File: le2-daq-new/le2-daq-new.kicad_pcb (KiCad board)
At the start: 2 copper layers, 161.3 x 88.4 mm, 11 parts, among them J1 PCIE_CONN, J2 PCIE_CONN, J3 PCIE_CONN, J4 PCIE_CONN, J5 Conn_01x02_Male, J6 TEST-POINT, J7 TEST-POINT, SW1 EN_HIGH, U1 ESP32-DEVKITC-32D

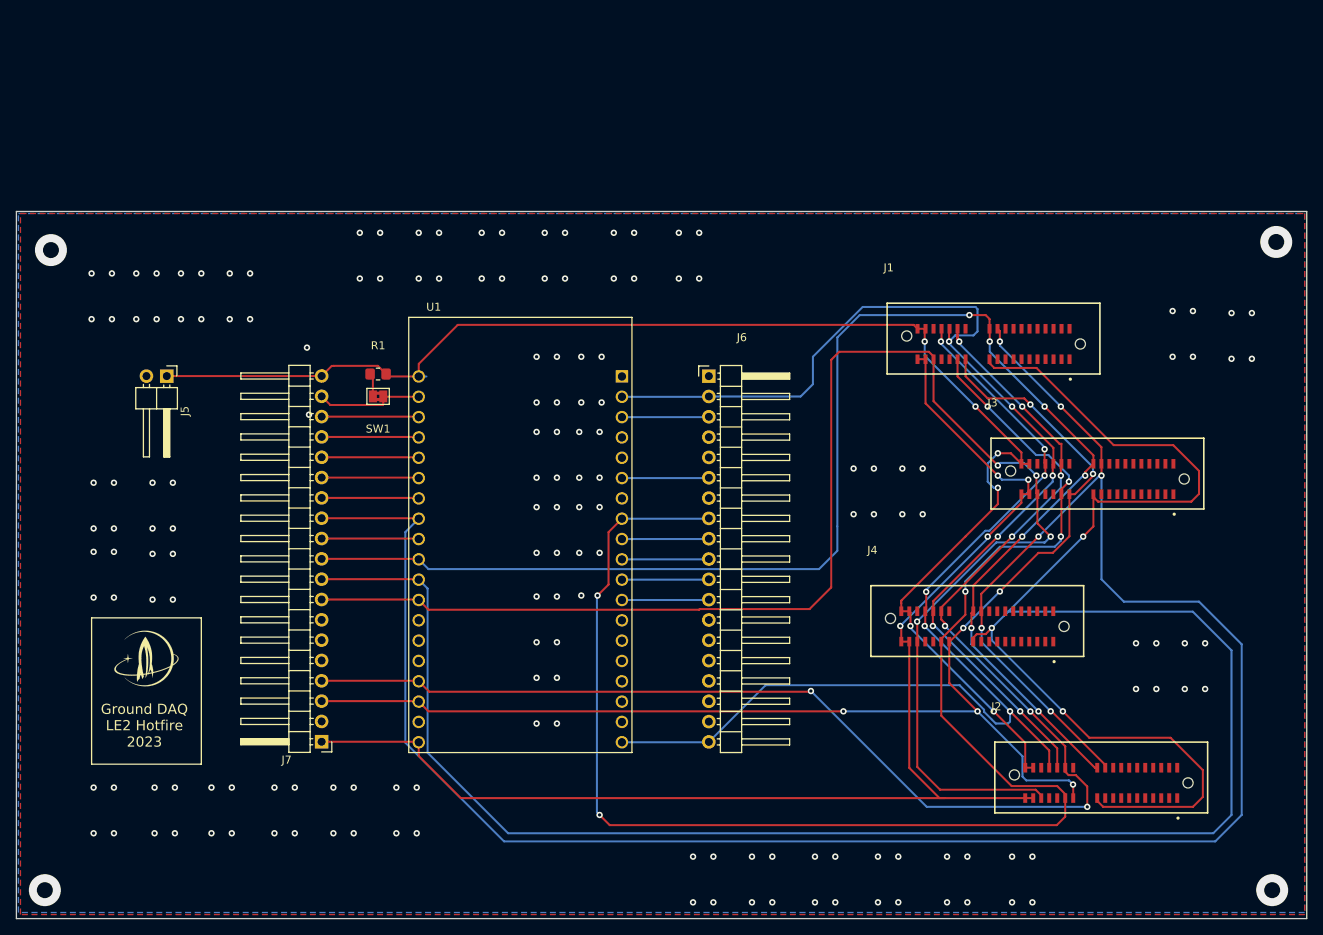
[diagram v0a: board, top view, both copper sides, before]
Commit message: done with daq layout FRFRFRF
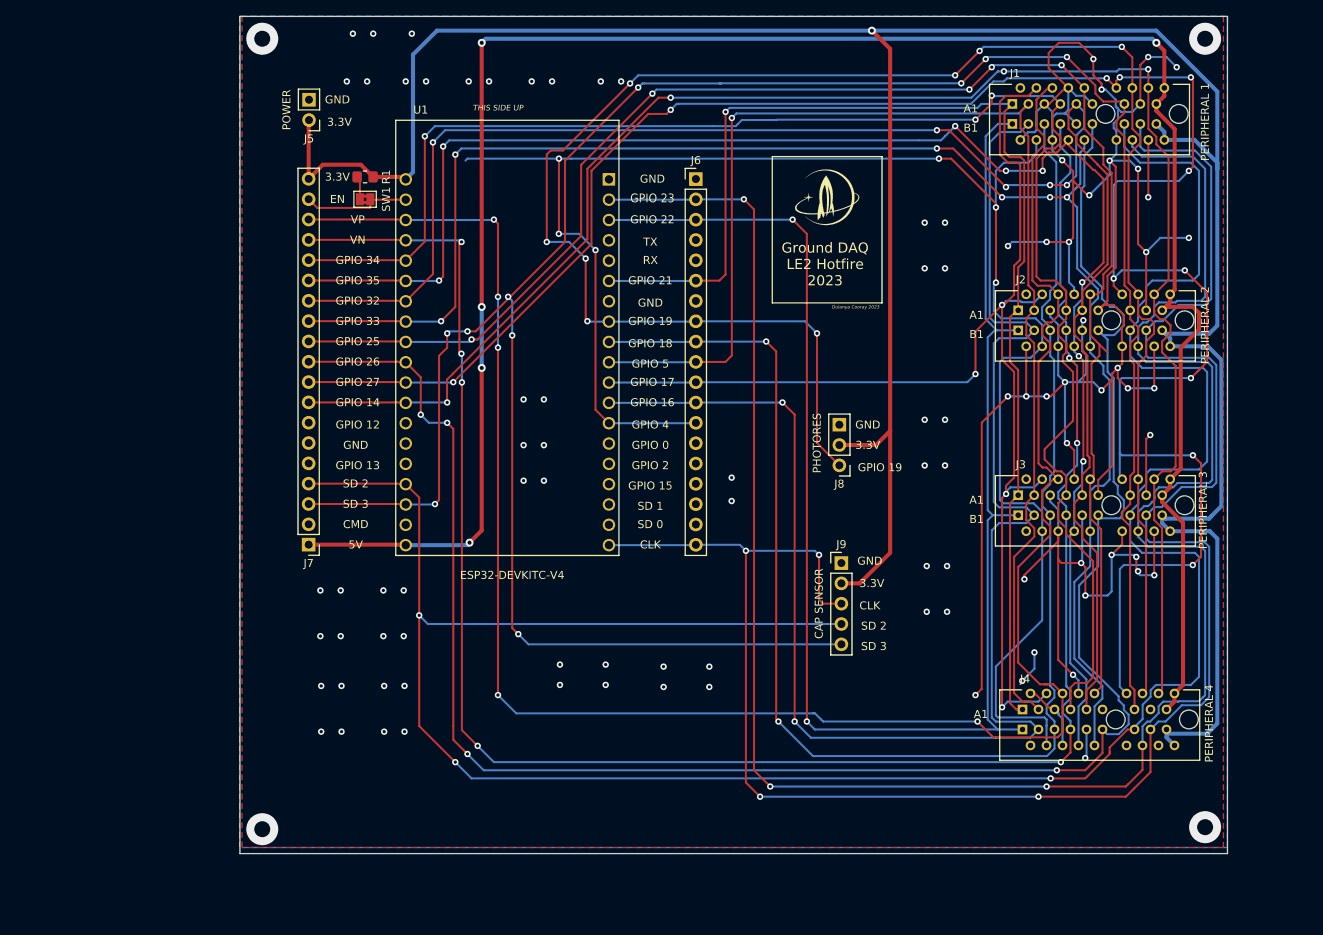
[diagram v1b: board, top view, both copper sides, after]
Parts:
- added J8: Conn_01x03_Male, Connector_PinHeader_2.54mm:PinHeader_1x03_P2.54mm_Vertical, F.Cu at (157.0, 89.4)
- added J9: Conn_01x05_Male, Connector_PinHeader_2.54mm:PinHeader_1x05_P2.54mm_Vertical, F.Cu at (157.2, 101.6)
- J1, J2, J3, J4: footprint PCIE-LP-01-01-F-DV-A-TR:SAMTEC_PCIE-LP-01-01-F-DV-A-TR -> AMPHENOL-PCIE-Socket:AMPHENOL_10018784-10210TLF
- J5: footprint Connector_PinHeader_2.54mm:PinHeader_1x02_P2.54mm_Horizontal -> Connector_PinHeader_2.54mm:PinHeader_1x02_P2.54mm_Vertical
- J6, J7: footprint Connector_PinHeader_2.54mm:PinHeader_1x19_P2.54mm_Horizontal -> Connector_PinHeader_2.54mm:PinHeader_1x19_P2.54mm_Vertical
- SW1: value EN_HIGH -> SW_Push
- moved G*** 102.8 mm to (155.4, 55.9)
- moved J2 57.8 mm to (191.0, 71.3)
- moved J5 36.6 mm to (90.7, 46.2), turned to 180 degrees
- moved J1 32.0 mm to (190.2, 45.5)
- moved J6 24.7 mm to (139.0, 53.6)
- moved SW1 24.7 mm to (97.7, 56.1)
- moved J7 24.7 mm to (90.6, 99.3)
- moved R1 24.7 mm to (97.7, 53.3)
- moved U1 24.7 mm to (115.5, 73.4)
- moved J4 20.8 mm to (191.5, 121.2)
- moved J3 3.71 mm to (191.0, 94.4)
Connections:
- J1 pad A01: (no net) -> RL SDA
- J1 pad A02: (no net) -> GND
- J1 pad A03: (no net) -> TC SDO
- J1 pad A04: (no net) -> TC SDI
- J1 pad A05: (no net) -> GND
- J1 pad A06: (no net) -> HX 1
- J1 pad A07: (no net) -> HX 3
- J1 pad A08: (no net) -> GND
- J1 pad A09: (no net) -> HX 5
- J1 pad A10: GND -> HX 7
- J1 pad A11: HX CLK -> GND
- J1 pad A12: CAP 2 -> HX CLK
- J1 pad A13: PHOTORES -> CAP 2
- J1 pad A14: GND -> PHOTORES
- J1 pad B01: (no net) -> RL SCL
- J1 pad B02: (no net) -> GND
- J1 pad B03: (no net) -> TC1 CS
- J1 pad B04: (no net) -> TC2 CS
- J1 pad B05: (no net) -> TC CLK
- J1 pad B06: (no net) -> GND
- J1 pad B07: (no net) -> HX 2
- J1 pad B08: (no net) -> HX 4
- J1 pad B09: (no net) -> GND
- J2 pad A01: (no net) -> RL SDA
- J2 pad A02: (no net) -> GND
- J2 pad A03: (no net) -> TC SDO
- J2 pad A04: (no net) -> TC SDI
- J2 pad A05: (no net) -> GND
- J2 pad A06: (no net) -> HX 1
- J2 pad A07: (no net) -> HX 3
- J2 pad A08: (no net) -> GND
- J2 pad A09: (no net) -> HX 5
- J2 pad A10: GND -> HX 7
- J2 pad A11: HX CLK -> GND
- J2 pad A12: CAP 2 -> HX CLK
- J2 pad A13: PHOTORES -> CAP 2
- J2 pad A14: GND -> PHOTORES
- J2 pad B01: (no net) -> RL SCL
- J2 pad B02: (no net) -> GND
- J2 pad B03: (no net) -> TC1 CS
- J2 pad B04: (no net) -> TC2 CS
- J2 pad B05: (no net) -> TC CLK
- J2 pad B06: (no net) -> GND
- J2 pad B07: (no net) -> HX 2
- J2 pad B08: (no net) -> HX 4
- J2 pad B09: (no net) -> GND
- J3 pad A01: (no net) -> RL SDA
- J3 pad A02: (no net) -> GND
- J3 pad A03: (no net) -> TC SDO
- J3 pad A04: (no net) -> TC SDI
- J3 pad A05: (no net) -> GND
- J3 pad A06: (no net) -> HX 1
- J3 pad A07: (no net) -> HX 3
- J3 pad A08: (no net) -> GND
- J3 pad A09: (no net) -> HX 5
- J3 pad A10: GND -> HX 7
- J3 pad A11: HX CLK -> GND
- J3 pad A12: CAP 2 -> HX CLK
- J3 pad A13: PHOTORES -> CAP 2
- J3 pad A14: GND -> PHOTORES
- J3 pad B01: (no net) -> RL SCL
- J3 pad B02: (no net) -> GND
- J3 pad B03: (no net) -> TC1 CS
- J3 pad B04: (no net) -> TC2 CS
- J3 pad B05: (no net) -> TC CLK
- J3 pad B06: (no net) -> GND
- J3 pad B07: (no net) -> HX 2
- J3 pad B08: (no net) -> HX 4
- J3 pad B09: (no net) -> GND
- J4 pad A01: (no net) -> RL SDA
- J4 pad A02: (no net) -> GND
- J4 pad A03: (no net) -> TC SDO
- J4 pad A04: (no net) -> TC SDI
- J4 pad A05: (no net) -> GND
- J4 pad A06: (no net) -> HX 1
- J4 pad A07: (no net) -> HX 3
- J4 pad A08: (no net) -> GND
- J4 pad A09: (no net) -> HX 5
- J4 pad A10: GND -> HX 7
- J4 pad A11: HX CLK -> GND
- J4 pad A12: CAP 2 -> HX CLK
- J4 pad A13: PHOTORES -> CAP 2
- J4 pad A14: GND -> PHOTORES
- J4 pad B01: (no net) -> RL SCL
- J4 pad B02: (no net) -> GND
- J4 pad B03: (no net) -> TC1 CS
- J4 pad B04: (no net) -> TC2 CS
- J4 pad B05: (no net) -> TC CLK
- J4 pad B06: (no net) -> GND
- J4 pad B07: (no net) -> HX 2
- J4 pad B08: (no net) -> HX 4
- J4 pad B09: (no net) -> GND
- J6 pad 10: TC1 CS -> TC SDO
- J6 pad 11: TC SDO -> TC SDI
- J6 pad 12: TC CLK -> TC1 CS
- J6 pad 13: unconnected-(J6-Pad13) -> TC2 CS
- J6 pad 9: TC2 CS -> TC CLK
- U1 pad 28: TC2 CS -> TC CLK
- U1 pad 29: TC1 CS -> TC SDO
- U1 pad 30: TC SDO -> TC SDI
- U1 pad 31: TC CLK -> TC1 CS
- U1 pad 32: unconnected-(U1-Pad32) -> TC2 CS
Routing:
- net GND: track 0.00 -> 385.6 mm, vias 167 -> 98
- net HX 1: track 12.2 -> 251.9 mm, vias 0 -> 5
- net HX 2: track 12.2 -> 242.6 mm, vias 0 -> 7
- net TC2 CS: track 10.9 -> 221.3 mm, vias 0 -> 6
- net HX 5: track 12.2 -> 214.0 mm, vias 0 -> 5
- net HX 3: track 12.2 -> 202.1 mm, vias 0 -> 3
- net RL SCL: track 10.9 -> 200.1 mm, vias 0 -> 2
- net HX 7: track 12.2 -> 200.6 mm, vias 0 -> 5
- net HX 4: track 12.2 -> 199.6 mm, vias 0 -> 8
- net TC1 CS: track 10.9 -> 195.1 mm, vias 0 -> 2
- net TC CLK: track 10.9 -> 186.7 mm, vias 0 -> 2
- net +3.3V: track 181.6 -> 347.5 mm, vias 6 -> 1
- net TC SDI: track 0.00 -> 158.9 mm, vias 0 -> 4
- net TC SDO: track 10.9 -> 164.6 mm, vias 0 -> 1
- net CAP 2: track 165.1 -> 308.7 mm, vias 7 -> 10
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- added copper zone on B.Cu, net GND
- removed copper zone on B.Cu, net (none)
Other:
- board size 161.3 x 88.4 mm -> 123.4 x 104.6 mm
- board text added: "3.3V"
- board text added: "5V"
- board text added: "CAP SENSOR"
- board text added: "CLK"
- board text added: "CMD"
- board text added: "Dulanya Cooray 2023"
- board text added: "EN"
- board text added: "ESP32-DEVKITC-V4"
- board text added: "GND"
- board text added: "GPIO 0"
- board text added: "GPIO 12"
- board text added: "GPIO 13"
- board text added: "GPIO 14"
- board text added: "GPIO 15"
- board text added: "GPIO 16"
- board text added: "GPIO 17"
- board text added: "GPIO 18"
- board text added: "GPIO 19"
- board text added: "GPIO 2"
- board text added: "GPIO 21"
- board text added: "GPIO 22"
- board text added: "GPIO 23"
- board text added: "GPIO 25"
- board text added: "GPIO 26"
- board text added: "GPIO 27"
- board text added: "GPIO 32"
- board text added: "GPIO 33"
- board text added: "GPIO 34"
- board text added: "GPIO 35"
- board text added: "GPIO 4"
- board text added: "GPIO 5"
- board text added: "PERIPHERAL 1"
- board text added: "PERIPHERAL 2"
- board text added: "PERIPHERAL 3"
- board text added: "PERIPHERAL 4"
- board text added: "PHOTORES"
- board text added: "POWER"
- board text added: "RX"
- board text added: "SD 0"
- board text added: "SD 1"
- board text added: "SD 2"
- board text added: "SD 3"
- board text added: "THIS SIDE UP"
- board text added: "TX"
- board text added: "VN"
- board text added: "VP"
